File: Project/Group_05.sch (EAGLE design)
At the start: 29 parts, among them J1 POWER_JACKPTH_LOCK, U1 +12v, U3 TCA9546A_SMD

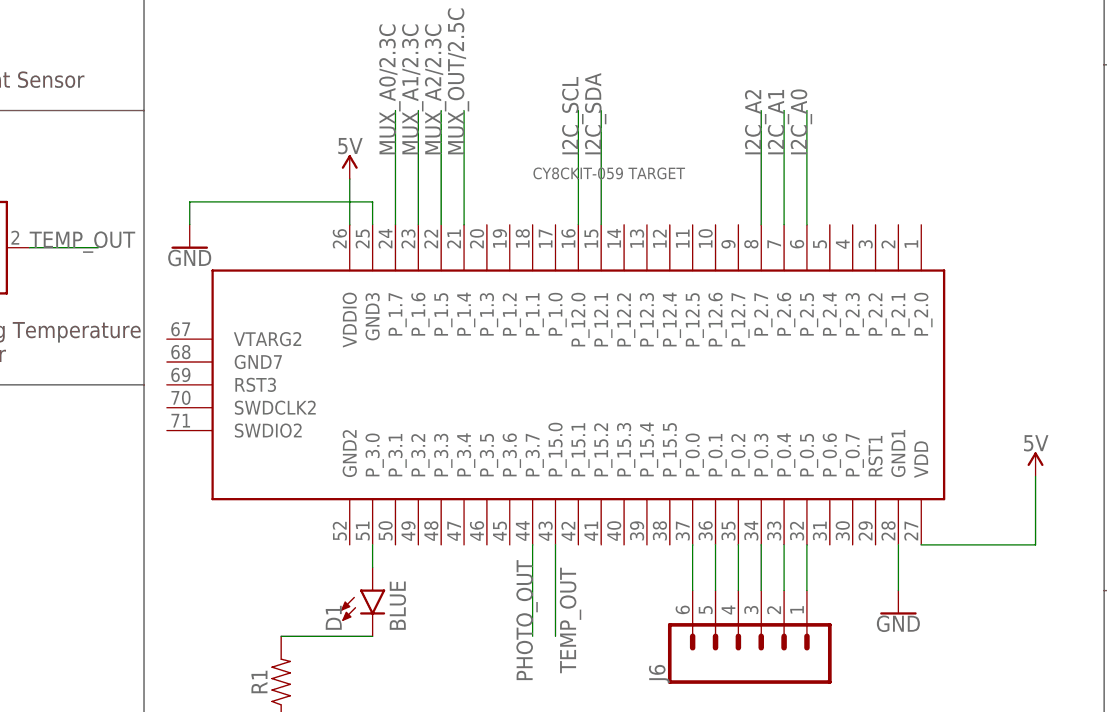
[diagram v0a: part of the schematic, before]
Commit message: Third schematic commit
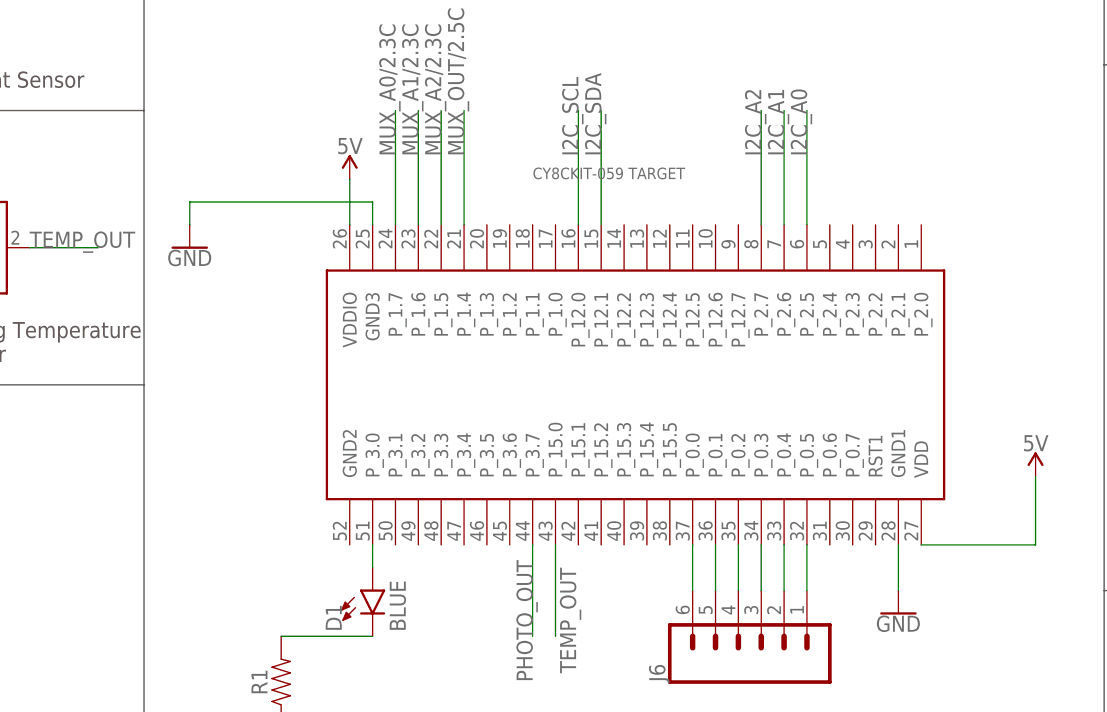
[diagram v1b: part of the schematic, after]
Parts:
- removed U$1: CY8CKIT-059_TARGET, CY8KIT-059:CY8CKIT-059_TARGET
- added U$3: CY8CKIT-059_TARGET_3, CY8KIT-059:CY8CKIT-059_TARGET_3
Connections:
- new net N$10: U$3.GND3
- new net N$11: U$3.VDDIO
- net 5V: now also U$3.VDD; no longer U$1.VDD, U$1.VDDIO
- net GND: now also U$3.GND1; no longer U$1.GND1, U$1.GND3
- net I2C_A0: now also U$3.P_2.5; no longer U$1.P_2.5
- net I2C_A1: now also U$3.P_2.6; no longer U$1.P_2.6
- net I2C_A2: now also U$3.P_2.7; no longer U$1.P_2.7
- net I2C_SCL: now also U$3.P_12.0; no longer U$1.P_12.0
- net I2C_SDA: now also U$3.P_12.1; no longer U$1.P_12.1
- net MUX_A0/2.3C: now also U$3.P_1.7; no longer U$1.P_1.7
- net MUX_A1/2.3C: now also U$3.P_1.6; no longer U$1.P_1.6
- net MUX_A2/2.3C: now also U$3.P_1.5; no longer U$1.P_1.5
- net MUX_OUT/2.5C: now also U$3.P_1.4; no longer U$1.P_1.4
- net N$1: now also U$3.P_0.0; no longer U$1.P_0.0
- net N$2: now also U$3.P_3.0; no longer U$1.P_3.0
- net N$5: now also U$3.P_0.1; no longer U$1.P_0.1
- net N$6: now also U$3.P_0.2; no longer U$1.P_0.2
- net N$7: now also U$3.P_0.3; no longer U$1.P_0.3
- net N$8: now also U$3.P_0.4; no longer U$1.P_0.4
- net N$9: now also U$3.P_0.5; no longer U$1.P_0.5
- net PHOTO_OUT: now also U$3.P_3.7; no longer U$1.P_3.7
- net TEMP_OUT: now also U$3.P_15.0; no longer U$1.P_15.0
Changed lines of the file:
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@@
 <parts>
 <part name="FRAME1" library="SparkFun-Aesthetics" deviceset="FRAME-A4L" device=""/>
-<part name="U$1" library="CY8KIT-059" deviceset="CY8CKIT-059_TARGET" device=""/>
 <part name="J1" library="SparkFun-Connectors" deviceset="POWER_JACK" device="PTH_LOCK"/>
 <part name="C2" library="SparkFun-Capacitors" deviceset="0.33UF/330NF" device="-0805-50V-10%" value="0.33µF"/>
@@
 <part name="J8" library="SparkFun-Connectors" deviceset="CONN_08" device="&quot;"/>
 <part name="U$2" library="Group_05_Library" deviceset="TMUX1208" device="_SMD"/>
+<part name="U$3" library="CY8KIT-059" deviceset="CY8CKIT-059_TARGET_3" device=""/>
 </parts>
 <sheets>
@@
 <attribute name="DESIGNER" x="226.26" y="6.35" size="2.54" layer="94" font="vector"/>
 </instance>
-<instance part="U$1" gate="G$1" x="40.64" y="71.12" smashed="yes"/>
 <instance part="J1" gate="G$1" x="15.24" y="162.56" smashed="yes">
 <attribute name="VALUE" x="5.08" y="172.72" size="1.778" layer="96" font="vector"/>
@@
 <attribute name="VALUE" x="218.44" y="50.8" size="2.54" layer="96"/>
 </instance>
+<instance part="U$3" gate="G$1" x="93.98" y="71.12" smashed="yes"/>
 </instances>
 <busses>
@@
 </segment>
 <segment>
-<pinref part="U$1" gate="G$1" pin="GND1"/>
 <pinref part="GND8" gate="1" pin="GND"/>
 <wire x1="124.46" y1="53.34" x2="124.46" y2="48.26" width="0.1524" layer="91"/>
+<pinref part="U$3" gate="G$1" pin="GND1"/>
 </segment>
 <segment>
@@
 <pinref part="GND7" gate="1" pin="GND"/>
 <wire x1="55.88" y1="33.02" x2="55.88" y2="27.94" width="0.1524" layer="91"/>
-</segment>
-<segment>
-<pinref part="GND10" gate="1" pin="GND"/>
-<wire x1="45.72" y1="88.9" x2="45.72" y2="91.44" width="0.1524" layer="91"/>
-<wire x1="45.72" y1="91.44" x2="66.04" y2="91.44" width="0.1524" layer="91"/>
-<pinref part="U$1" gate="G$1" pin="GND3"/>
-<wire x1="66.04" y1="91.44" x2="66.04" y2="88.9" width="0.1524" layer="91"/>
 </segment>
 <segment>
@@
 </segment>
 <segment>
-<pinref part="U$1" gate="G$1" pin="VDD"/>
 <wire x1="127" y1="53.34" x2="139.7" y2="53.34" width="0.1524" layer="91"/>
 <wire x1="139.7" y1="53.34" x2="139.7" y2="60.96" width="0.1524" layer="91"/>
 <pinref part="SUPPLY8" gate="G$1" pin="5V"/>
-</segment>
-<segment>
-<pinref part="SUPPLY9" gate="G$1" pin="5V"/>
-<pinref part="U$1" gate="G$1" pin="VDDIO"/>
-<wire x1="63.5" y1="93.98" x2="63.5" y2="88.9" width="0.1524" layer="91"/>
+<pinref part="U$3" gate="G$1" pin="VDD"/>
 </segment>
 <segment>
@@
 </segment>
 <segment>
-<pinref part="U$1" gate="G$1" pin="P_3.7"/>
 <wire x1="83.82" y1="53.34" x2="83.82" y2="43.18" width="0.1524" layer="91"/>
 <label x="83.82" y="38.1" size="1.778" layer="95" rot="R90"/>
+<pinref part="U$3" gate="G$1" pin="P_3.7"/>
 </segment>
 </net>
@@
 </segment>
 <segment>
-<pinref part="U$1" gate="G$1" pin="P_15.0"/>
 <wire x1="86.36" y1="53.34" x2="86.36" y2="43.18" width="0.1524" layer="91"/>
 <label x="86.868" y="50.8" size="1.778" layer="95" rot="R270"/>
+<pinref part="U$3" gate="G$1" pin="P_15.0"/>
 </segment>
 </net>
@@
 </segment>
 <segment>
-<pinref part="U$1" gate="G$1" pin="P_12.1"/>
 <wire x1="91.44" y1="88.9" x2="91.44" y2="101.6" width="0.1524" layer="91"/>
 <label x="91.44" y="96.52" size="1.778" layer="95" rot="R90"/>
+<pinref part="U$3" gate="G$1" pin="P_12.1"/>
 </segment>
 </net>
@@
 </segment>
 <segment>
-<pinref part="U$1" gate="G$1" pin="P_12.0"/>
 <wire x1="88.9" y1="88.9" x2="88.9" y2="101.6" width="0.1524" layer="91"/>
 <label x="88.9" y="96.52" size="1.778" layer="95" rot="R90"/>
+<pinref part="U$3" gate="G$1" pin="P_12.0"/>
 </segment>
 </net>
@@
 </segment>
 <segment>
-<pinref part="U$1" gate="G$1" pin="P_2.5"/>
 <wire x1="114.3" y1="88.9" x2="114.3" y2="101.6" width="0.1524" layer="91"/>
 <label x="114.3" y="96.52" size="1.778" layer="95" rot="R90"/>
+<pinref part="U$3" gate="G$1" pin="P_2.5"/>
 </segment>
 </net>
@@
 </segment>
 <segment>
-<pinref part="U$1" gate="G$1" pin="P_2.6"/>
 <wire x1="111.76" y1="88.9" x2="111.76" y2="101.6" width="0.1524" layer="91"/>
 <label x="111.76" y="96.52" size="1.778" layer="95" rot="R90"/>
+<pinref part="U$3" gate="G$1" pin="P_2.6"/>
 </segment>
 </net>
@@
 </segment>
 <segment>
-<pinref part="U$1" gate="G$1" pin="P_2.7"/>
 <wire x1="109.22" y1="88.9" x2="109.22" y2="101.6" width="0.1524" layer="91"/>
 <label x="109.22" y="96.52" size="1.778" layer="95" rot="R90"/>
+<pinref part="U$3" gate="G$1" pin="P_2.7"/>
 </segment>
 </net>
@@
 <net name="N$2" class="0">
 <segment>
-<pinref part="U$1" gate="G$1" pin="P_3.0"/>
 <pinref part="D1" gate="G$1" pin="A"/>
 <wire x1="66.04" y1="53.34" x2="66.04" y2="50.8" width="0.1524" layer="91"/>
+<pinref part="U$3" gate="G$1" pin="P_3.0"/>
 </segment>
 </net>
@@
 <net name="N$1" class="0">
 <segment>
-<pinref part="U$1" gate="G$1" pin="P_0.0"/>
 <pinref part="J6" gate="G$1" pin="6"/>
 <wire x1="101.6" y1="53.34" x2="101.6" y2="48.26" width="0.1524" layer="91"/>
+<pinref part="U$3" gate="G$1" pin="P_0.0"/>
 </segment>
 </net>
 <net name="N$5" class="0">
 <segment>
-<pinref part="U$1" gate="G$1" pin="P_0.1"/>
 <pinref part="J6" gate="G$1" pin="5"/>
 <wire x1="104.14" y1="53.34" x2="104.14" y2="48.26" width="0.1524" layer="91"/>
+<pinref part="U$3" gate="G$1" pin="P_0.1"/>
 </segment>
 </net>
 <net name="N$6" class="0">
 <segment>
-<pinref part="U$1" gate="G$1" pin="P_0.2"/>
 <pinref part="J6" gate="G$1" pin="4"/>
 <wire x1="106.68" y1="53.34" x2="106.68" y2="48.26" width="0.1524" layer="91"/>
+<pinref part="U$3" gate="G$1" pin="P_0.2"/>
 </segment>
 </net>
 <net name="N$7" class="0">
 <segment>
-<pinref part="U$1" gate="G$1" pin="P_0.3"/>
 <pinref part="J6" gate="G$1" pin="3"/>
 <wire x1="109.22" y1="53.34" x2="109.22" y2="48.26" width="0.1524" layer="91"/>
+<pinref part="U$3" gate="G$1" pin="P_0.3"/>
 </segment>
 </net>
 <net name="N$8" class="0">
 <segment>
-<pinref part="U$1" gate="G$1" pin="P_0.4"/>
 <pinref part="J6" gate="G$1" pin="2"/>
 <wire x1="111.76" y1="53.34" x2="111.76" y2="48.26" width="0.1524" layer="91"/>
+<pinref part="U$3" gate="G$1" pin="P_0.4"/>
 </segment>
 </net>
 <net name="N$9" class="0">
 <segment>
-<pinref part="U$1" gate="G$1" pin="P_0.5"/>
 <pinref part="J6" gate="G$1" pin="1"/>
 <wire x1="114.3" y1="53.34" x2="114.3" y2="48.26" width="0.1524" layer="91"/>
+<pinref part="U$3" gate="G$1" pin="P_0.5"/>
 </segment>
 </net>
 <net name="MUX_A0/2.3C" class="0">
 <segment>
-<pinref part="U$1" gate="G$1" pin="P_1.7"/>
 <wire x1="68.58" y1="88.9" x2="68.58" y2="101.6" width="0.1524" layer="91"/>
 <label x="68.58" y="96.52" size="1.778" layer="95" rot="R90"/>
+<pinref part="U$3" gate="G$1" pin="P_1.7"/>
 </segment>
 </net>
 <net name="MUX_A1/2.3C" class="0">
 <segment>
-<pinref part="U$1" gate="G$1" pin="P_1.6"/>
 <wire x1="71.12" y1="88.9" x2="71.12" y2="101.6" width="0.1524" layer="91"/>
 <label x="71.12" y="96.52" size="1.778" layer="95" rot="R90"/>
+<pinref part="U$3" gate="G$1" pin="P_1.6"/>
 </segment>
 </net>
 <net name="MUX_A2/2.3C" class="0">
 <segment>
-<pinref part="U$1" gate="G$1" pin="P_1.5"/>
 <wire x1="73.66" y1="88.9" x2="73.66" y2="101.6" width="0.1524" layer="91"/>
 <label x="73.66" y="96.52" size="1.778" layer="95" rot="R90"/>
+<pinref part="U$3" gate="G$1" pin="P_1.5"/>
 </segment>
 </net>
 <net name="MUX_OUT/2.5C" class="0">
 <segment>
-<pinref part="U$1" gate="G$1" pin="P_1.4"/>
 <wire x1="76.2" y1="88.9" x2="76.2" y2="101.6" width="0.1524" layer="91"/>
 <label x="76.2" y="96.52" size="1.778" layer="95" rot="R90"/>
+<pinref part="U$3" gate="G$1" pin="P_1.4"/>
 </segment>
 </net>
@@
 </segment>
 </net>
+<net name="N$10" class="0">
+<segment>
+<pinref part="GND10" gate="1" pin="GND"/>
+<wire x1="45.72" y1="88.9" x2="45.72" y2="91.44" width="0.1524" layer="91"/>
+<wire x1="45.72" y1="91.44" x2="66.04" y2="91.44" width="0.1524" layer="91"/>
+<wire x1="66.04" y1="91.44" x2="66.04" y2="88.9" width="0.1524" layer="91"/>
+<pinref part="U$3" gate="G$1" pin="GND3"/>
+</segment>
+</net>
+<net name="N$11" class="0">
+<segment>
+<pinref part="SUPPLY9" gate="G$1" pin="5V"/>
+<wire x1="63.5" y1="93.98" x2="63.5" y2="88.9" width="0.1524" layer="91"/>
+<pinref part="U$3" gate="G$1" pin="VDDIO"/>
+</segment>
+</net>

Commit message: 4th schematic commit (completed?)
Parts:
- J8: device SparkFun-Connectors:CONN_08" -> SparkFun-Connectors:CONN_08LOCK
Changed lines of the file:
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@@
 <part name="GND14" library="SparkFun-PowerSymbols" deviceset="GND" device=""/>
 <part name="SUPPLY11" library="SparkFun-PowerSymbols" deviceset="5V" device=""/>
-<part name="J8" library="SparkFun-Connectors" deviceset="CONN_08" device="&quot;"/>
 <part name="U$2" library="Group_05_Library" deviceset="TMUX1208" device="_SMD"/>
 <part name="U$3" library="CY8KIT-059" deviceset="CY8CKIT-059_TARGET_3" device=""/>
+<part name="J8" library="SparkFun-Connectors" deviceset="CONN_08" device="LOCK"/>
 </parts>
 <sheets>
@@
 <attribute name="VALUE" x="241.3" y="86.614" size="1.778" layer="96" align="bottom-center"/>
 </instance>
+<instance part="U$2" gate="G$1" x="218.44" y="81.28" smashed="yes">
+<attribute name="NAME" x="228.6" y="96.52" size="2.54" layer="95"/>
+<attribute name="VALUE" x="218.44" y="50.8" size="2.54" layer="96"/>
+</instance>
+<instance part="U$3" gate="G$1" x="93.98" y="71.12" smashed="yes"/>
 <instance part="J8" gate="G$1" x="187.96" y="55.88" smashed="yes">
 <attribute name="VALUE" x="182.88" y="43.434" size="1.778" layer="96" font="vector"/>
 <attribute name="NAME" x="182.88" y="69.088" size="1.778" layer="95" font="vector"/>
 </instance>
-<instance part="U$2" gate="G$1" x="218.44" y="81.28" smashed="yes">
-<attribute name="NAME" x="228.6" y="96.52" size="2.54" layer="95"/>
-<attribute name="VALUE" x="218.44" y="50.8" size="2.54" layer="96"/>
-</instance>
-<instance part="U$3" gate="G$1" x="93.98" y="71.12" smashed="yes"/>
 </instances>
 <busses>
@@
 <net name="S1" class="0">
 <segment>
-<pinref part="J8" gate="G$1" pin="8"/>
 <wire x1="193.04" y1="66.04" x2="198.12" y2="66.04" width="0.1524" layer="91"/>
 <label x="198.12" y="66.04" size="1.778" layer="95"/>
+<pinref part="J8" gate="G$1" pin="8"/>
 </segment>
 <segment>
@@
 <net name="S2" class="0">
 <segment>
-<pinref part="J8" gate="G$1" pin="7"/>
 <wire x1="193.04" y1="63.5" x2="198.12" y2="63.5" width="0.1524" layer="91"/>
 <label x="198.12" y="63.5" size="1.778" layer="95"/>
+<pinref part="J8" gate="G$1" pin="7"/>
 </segment>
 <segment>
@@
 <net name="S3" class="0">
 <segment>
-<pinref part="J8" gate="G$1" pin="6"/>
 <wire x1="193.04" y1="60.96" x2="198.12" y2="60.96" width="0.1524" layer="91"/>
 <label x="198.12" y="60.96" size="1.778" layer="95"/>
+<pinref part="J8" gate="G$1" pin="6"/>
 </segment>
 <segment>
@@
 <net name="S4" class="0">
 <segment>
-<pinref part="J8" gate="G$1" pin="5"/>
 <wire x1="193.04" y1="58.42" x2="198.12" y2="58.42" width="0.1524" layer="91"/>
 <label x="198.12" y="58.42" size="1.778" layer="95"/>
+<pinref part="J8" gate="G$1" pin="5"/>
 </segment>
 <segment>
@@
 <net name="S5" class="0">
 <segment>
-<pinref part="J8" gate="G$1" pin="4"/>
 <wire x1="193.04" y1="55.88" x2="198.12" y2="55.88" width="0.1524" layer="91"/>
 <label x="198.12" y="55.88" size="1.778" layer="95"/>
+<pinref part="J8" gate="G$1" pin="4"/>
 </segment>
 <segment>
@@
 <net name="S6" class="0">
 <segment>
-<pinref part="J8" gate="G$1" pin="3"/>
 <wire x1="193.04" y1="53.34" x2="198.12" y2="53.34" width="0.1524" layer="91"/>
 <label x="198.12" y="53.34" size="1.778" layer="95"/>
+<pinref part="J8" gate="G$1" pin="3"/>
 </segment>
 <segment>
@@
 <net name="S7" class="0">
 <segment>
-<pinref part="J8" gate="G$1" pin="2"/>
 <wire x1="193.04" y1="50.8" x2="198.12" y2="50.8" width="0.1524" layer="91"/>
 <label x="198.12" y="50.8" size="1.778" layer="95"/>
+<pinref part="J8" gate="G$1" pin="2"/>
 </segment>
 <segment>
@@
 <net name="S8" class="0">
 <segment>
-<pinref part="J8" gate="G$1" pin="1"/>
 <wire x1="193.04" y1="48.26" x2="198.12" y2="48.26" width="0.1524" layer="91"/>
 <label x="198.12" y="48.26" size="1.778" layer="95"/>
-</segment>
-<segment>
+<pinref part="J8" gate="G$1" pin="1"/>
+</segment>
+<segment>
